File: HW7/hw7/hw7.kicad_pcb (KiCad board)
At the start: 2 copper layers, 16 parts, among them J1 Jack-DC, J2 Conn_01x02_Pin, J3 Screw_Terminal_01x02, K1 SANYOU_SRD_Form_C, Q1 BC337-40, U1 817C

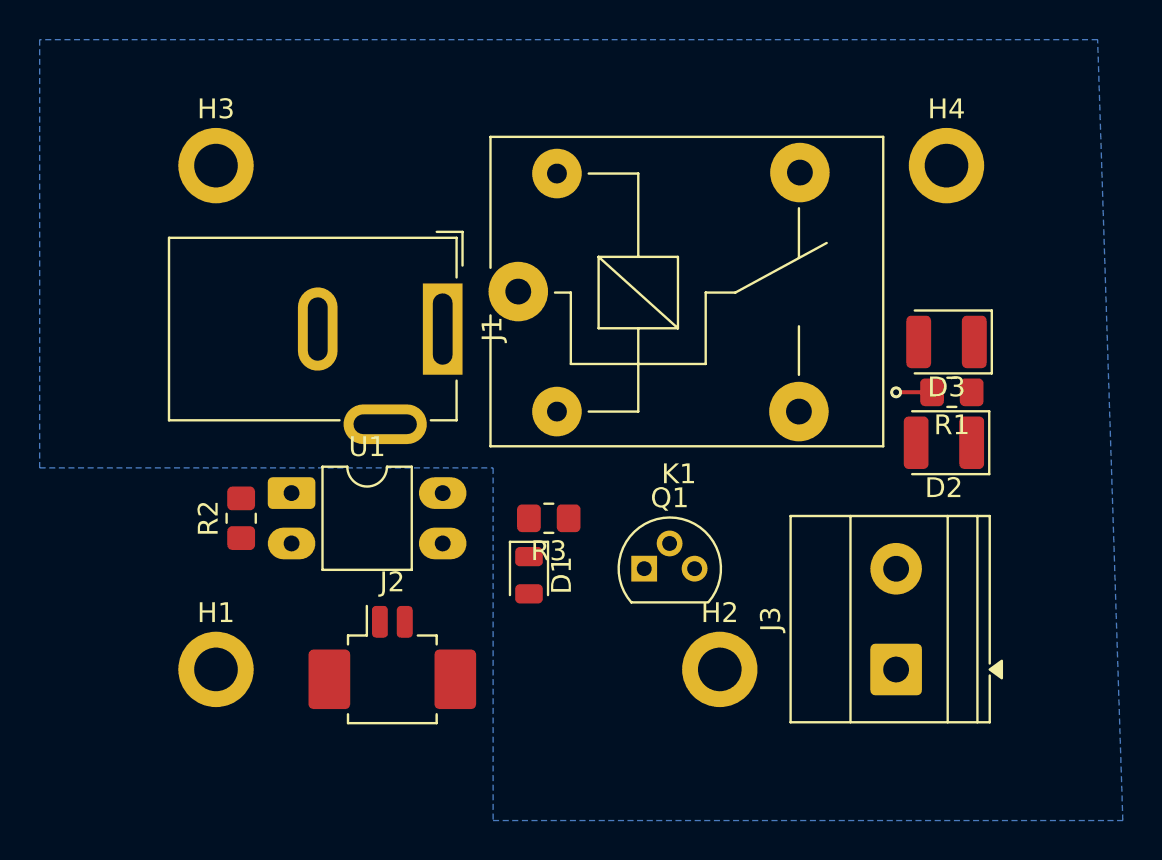
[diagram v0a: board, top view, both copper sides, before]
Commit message: HW7-HW8
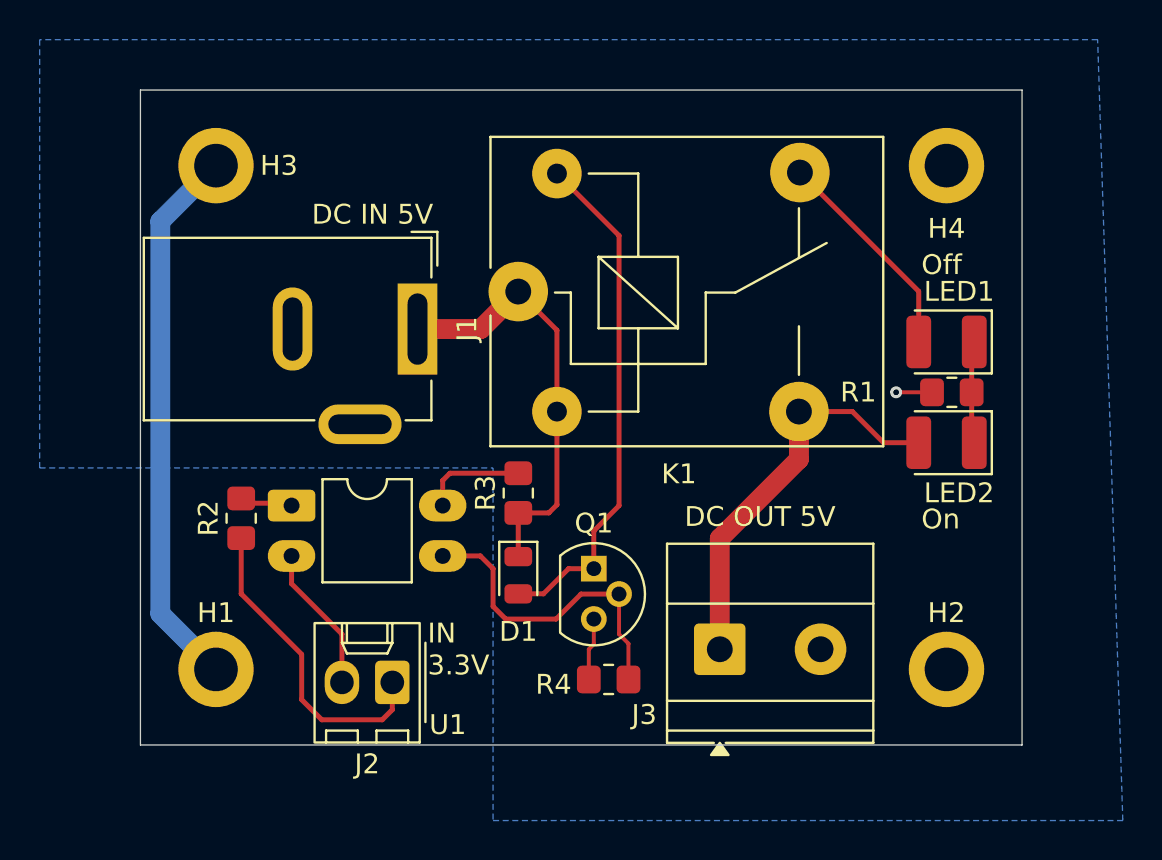
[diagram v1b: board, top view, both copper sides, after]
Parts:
- added R4: 10к, Resistor_SMD:R_0805_2012Metric_Pad1.20x1.40mm_HandSolder, F.Cu at (121.4, 65.3)
- J2: footprint Connector_Molex:Molex_PicoBlade_53261-0271_1x02-1MP_P1.25mm_Horizontal -> Connector_Molex:Molex_KK-254_AE-6410-02A_1x02_P2.54mm_Vertical
- LED1: renamed from D3; value Green -> Red
- LED2: renamed from D2; value Red -> Green
- moved H2 11.4 mm to (138.4, 64.8)
- moved J3 8.95 mm to (127.0, 63.8), turned to 0 degrees
- moved Q1 2.54 mm to (120.7, 59.7), turned to -90 degrees
- moved R3 2.00 mm to (116.8, 55.9), turned to 90 degrees
- moved J1 1.27 mm to (111.8, 47.6)
- moved J2 0.66 mm to (110.5, 65.4), turned to 180 degrees
- moved U1 0.63 mm to (105.4, 56.5)
- moved D1 0.54 mm to (116.8, 60.0)
- moved LED2 0.13 mm to (138.4, 53.3)
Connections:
- H1 pad 1: (no net) -> GND
- H2 pad 1: (no net) -> GND
- H3 pad 1: (no net) -> GND
- H4 pad 1: (no net) -> GND
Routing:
- net GND: track 1.81 -> 32.7 mm
- net Net-(D1-A): track 0.00 -> 25.4 mm
- net +5V: track 0.00 -> 21.7 mm
- net Net-(J3-Pin_1): track 0.00 -> 20.2 mm
- net Net-(Q1-B): track 0.00 -> 16.4 mm
- net VS: track 0.00 -> 16.0 mm
- net Net-(LED1-A): track 0.00 -> 11.0 mm
- net GNDS: track 0.00 -> 7.43 mm
- net Net-(R3-Pad2): track 0.00 -> 5.23 mm
- net Net-(LED1-K): track 0.00 -> 5.13 mm
- net Net-(R2-Pad2): track 0.00 -> 2.69 mm
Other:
- board outline added: 44.5 x 33 mm
- board text added: "DC IN 5V"
- board text added: "DC OUT 5V"
- board text added: "IN 3.3V"
- board text added: "Off"
- board text added: "On"
